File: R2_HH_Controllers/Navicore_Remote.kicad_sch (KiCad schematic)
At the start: 56 parts, among them IC1 E22-900M22S, J1 USB4105-GF-A, J2 S2B-PH-SM4-TB_LF__SN_, SW1 SW_Push, SW10 Boot, SW11 PCM12SMTR, SW2 SW_Push, SW3 SW_Push, SW4 SW_Push, SW5 SW_Push, SW6 SW_Push, SW7 SW_Push, SW8 SW_Push, SW9 Reset, U1 AP2112K-3.3, U2 ESP32-S3-MINI-1, U3 BQ24074RGT, U4 USBLC6-2SC6

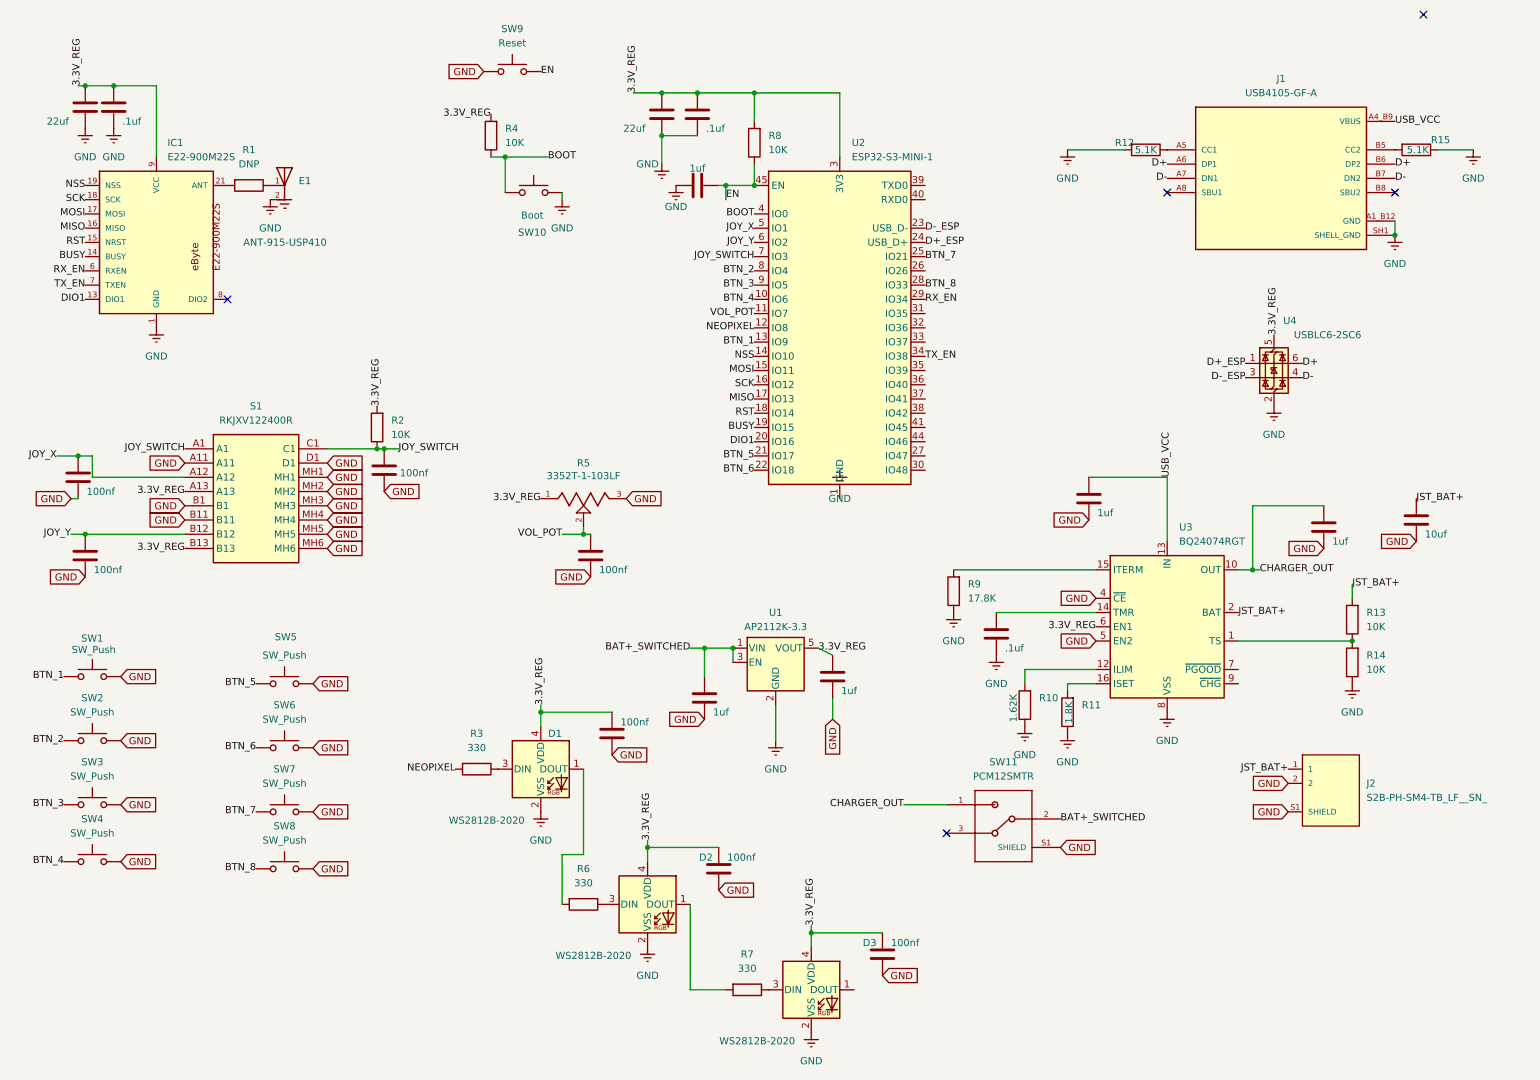
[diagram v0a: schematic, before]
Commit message: up
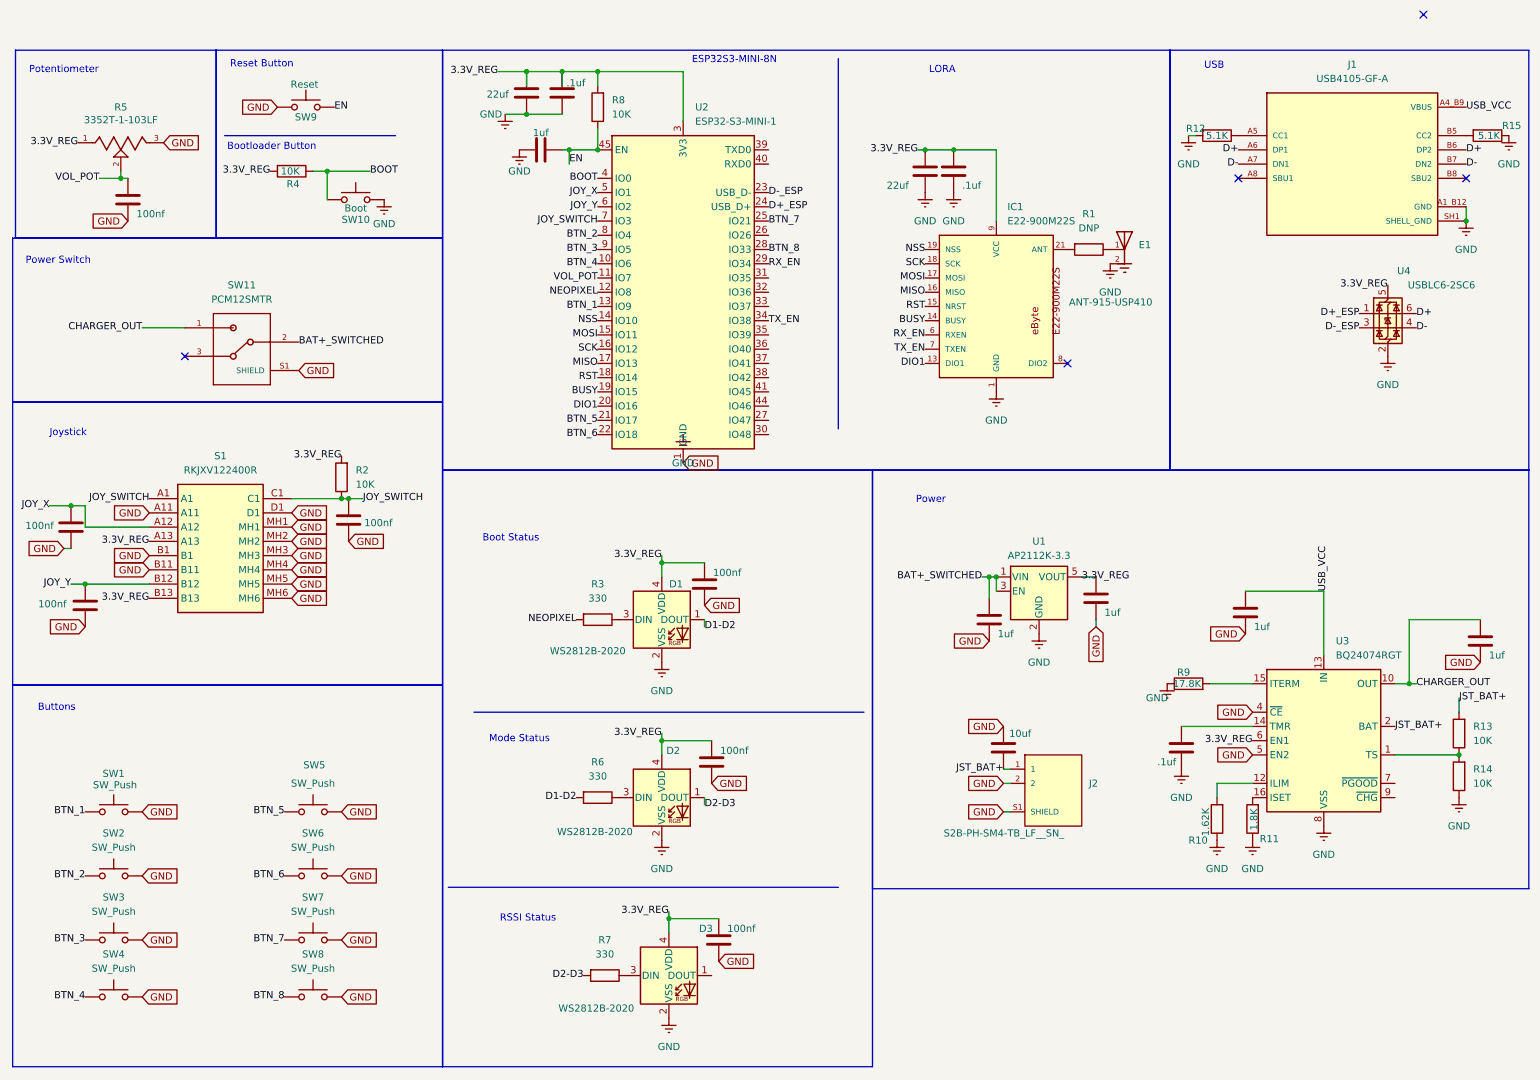
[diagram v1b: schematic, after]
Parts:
- E1: footprint custom:XDCR_ANT-915-USP410 -> 01-Custom:XDCR_ANT-915-USP410
- IC1: footprint custom:E22-900M22S -> 01-Custom:E22-900M22S
- SW1, SW2, SW3, SW4, SW5, SW6, SW7, SW8: footprint 01-Custom:TL3360CF185Q -> 01-Custom:SW_TL3360AF185Q
- U2: footprint 01-Custom:ESP32-S2-MINI-1 -> 01-Custom:XCVR_ESP32-S3-MINI-1-N8
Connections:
- net GND: now also C18.2, U2.1 (GND), U2.2 (GND), U2.42 (GND), U2.43 (GND), U2.46 (GND), U2.47 (GND), U2.48 (GND), U2.49 (GND), U2.50 (GND), U2.51 (GND), U2.52 (GND), U2.53 (GND), U2.54 (GND), U2.55 (GND), U2.56 (GND), U2.57 (GND), U2.58 (GND), U2.59 (GND), U2.60 (GND), U2.61 (GND), U2.62 (GND), U2.63 (GND), U2.64 (GND), U2.65 (GND); no longer C18.1
- net JST_BAT+: now also C18.1; no longer C18.2
- net D1-D2: now reaches D1.1 (DOUT), R6.2
- net D2-D3: now reaches D2.1 (DOUT), R7.2
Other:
- note added: "Boot Status"
- note added: "Bootloader Button"
- note added: "Buttons"
- note added: "ESP32S3-MINI-8N"
- note added: "Joystick"
- note added: "LORA"
- note added: "Mode Status"
- note added: "Potentiometer"
- note added: "Power"
- note added: "Power Switch"
- note added: "RSSI Status"
- note added: "Reset Button"
- note added: "USB"
- moved on the sheet: D1, D2, D3, E1, IC1, J1, J2, R1, R10, R11, R12, R13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
